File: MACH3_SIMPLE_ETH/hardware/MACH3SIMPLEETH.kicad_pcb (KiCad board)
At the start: 4 copper layers, 210 x 155 mm, 337 parts, among them J101 SENSORS / 24V IN, J201 USB-C, J202 SWD, J203 microSD, J301 HR911105A, J401 X axis, J402 Y axis, J403 Z axis, J404 A axis, J405 B axis, J406 C axis, J407 U axis, J408 V axis, J409 ENABLE, J501 LIMITS X Y Z A B C U V, J502 EST HLD RUN PRB, J503 THC AOK UP DN, J601 EXPANSION, J611 Relay A, J612 Relay B, J613 Relay C, J614 Relay D, J615 Relay E, J616 Relay F, J701 VFD, J801 RS485 A B GND, J802 HW ICSP, J803 MPG PENDANT, K601 JQC-3FF-024-1Z, K602 JQC-3FF-024-1Z, K603 JQC-3FF-024-1Z, K604 JQC-3FF-024-1Z, K605 JQC-3FF-024-1Z, K606 JQC-3FF-024-1Z, Q601 AO3400A, Q602 AO3400A, Q603 AO3400A, Q604 AO3400A, Q605 AO3400A, Q606 AO3400A, SW201 RESET, SW202 BOOTSEL, U101 LM2596S-5, U102 AP7361C-33E, U201 RP2350B, U202 W25Q128JVS, U203 USBLC6-2SC6, U301 W5500, U401 74ACT245, U402 74ACT245, U403 74ACT245, U501 PC847, U502 PC847, U503 PC847, U504 PC847, U601 MCP23017-E/SO, U701 74HCT14, U702 PC847, U703 B2412S-1WR3, U704 78L05, U705 LM358, U801 MAX3485ESA, U802 ATmega328P-AU, Y201 12MHz ABM8-272-T3, Y301 25MHz 18pF, Y801 8MHz

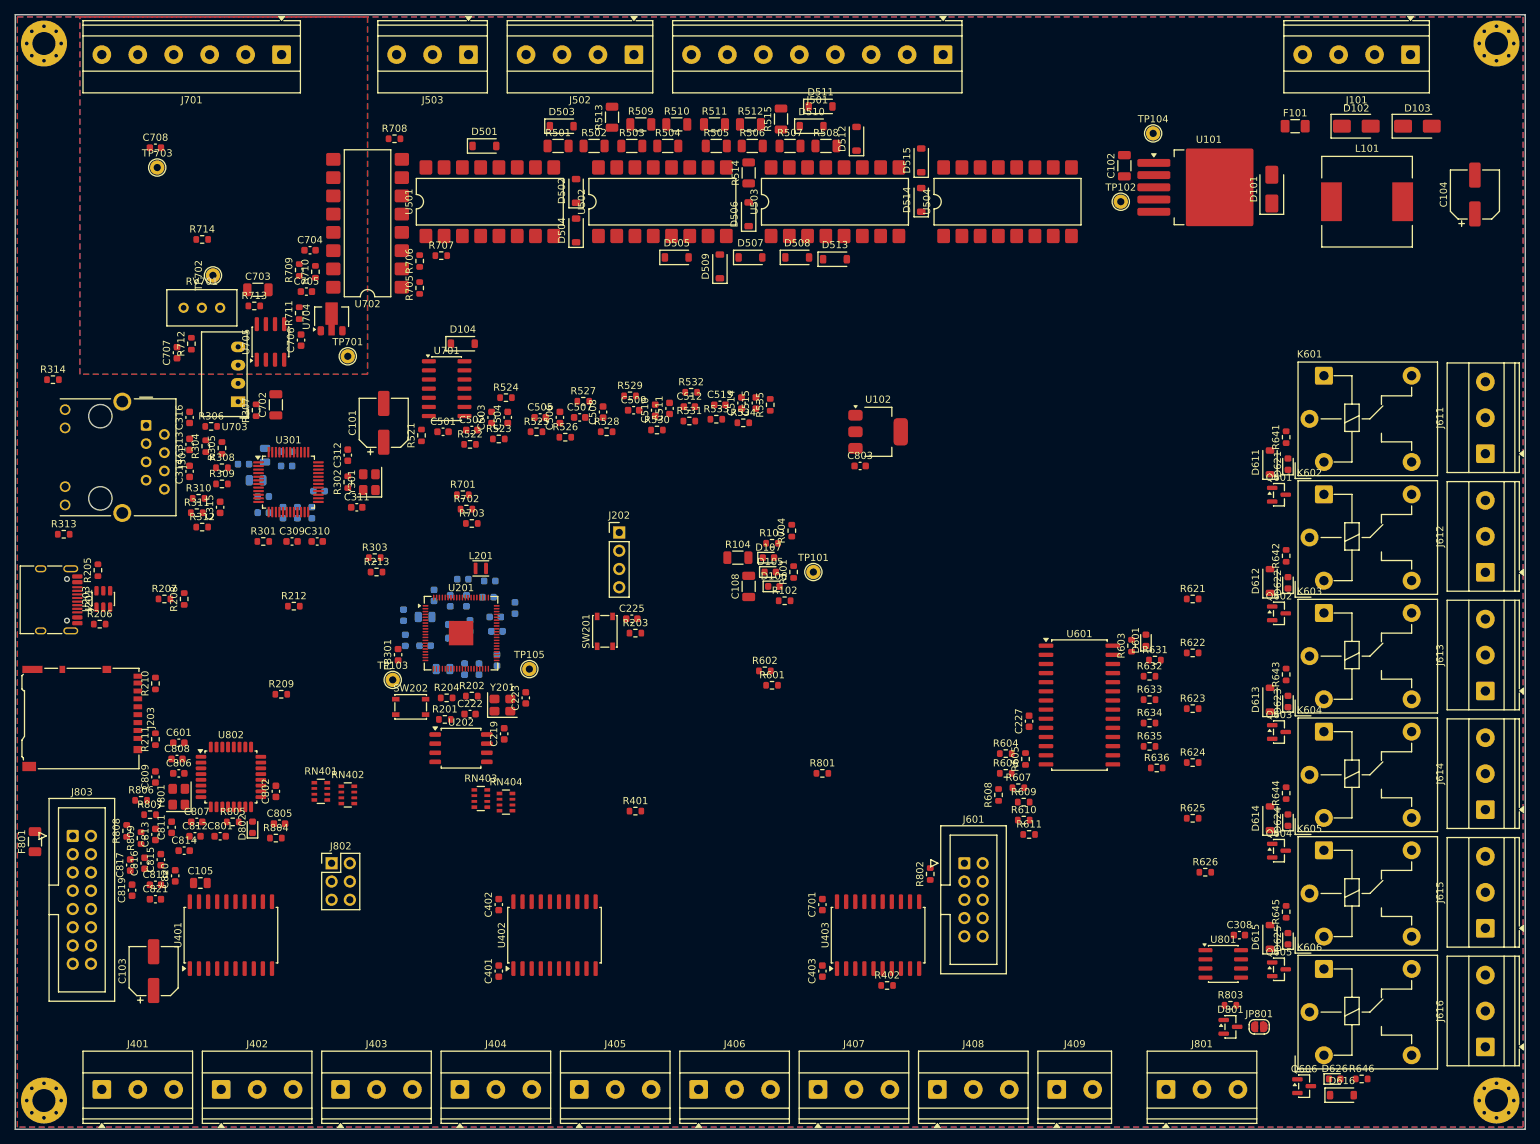
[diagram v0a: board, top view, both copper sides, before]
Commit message: MACH3-SIMPLE-ETH: routing pass 1 imported and filled
Freerouting pass 1 (board nets, VFD corner kept out): 1 h 40 min, 40
passes. After the zone fill 44 connections remain: 29 on the VFD side
(pass 2's job) and 15 others - 7 GND pins inside the RP2350B/W5500 fanout,
3 CHASSIS, 3 VBUS, 2 +3V3. Most of the 91 Freerouting reported were GND
pads that reach the ground pours once they are filled.

Co-Authored-By: Claude Opus 5.5 <noreply@anthropic.com>
Claude-Session: https://claude.ai/code/session_01MByiLT2xCcbGPkgCYQy33q
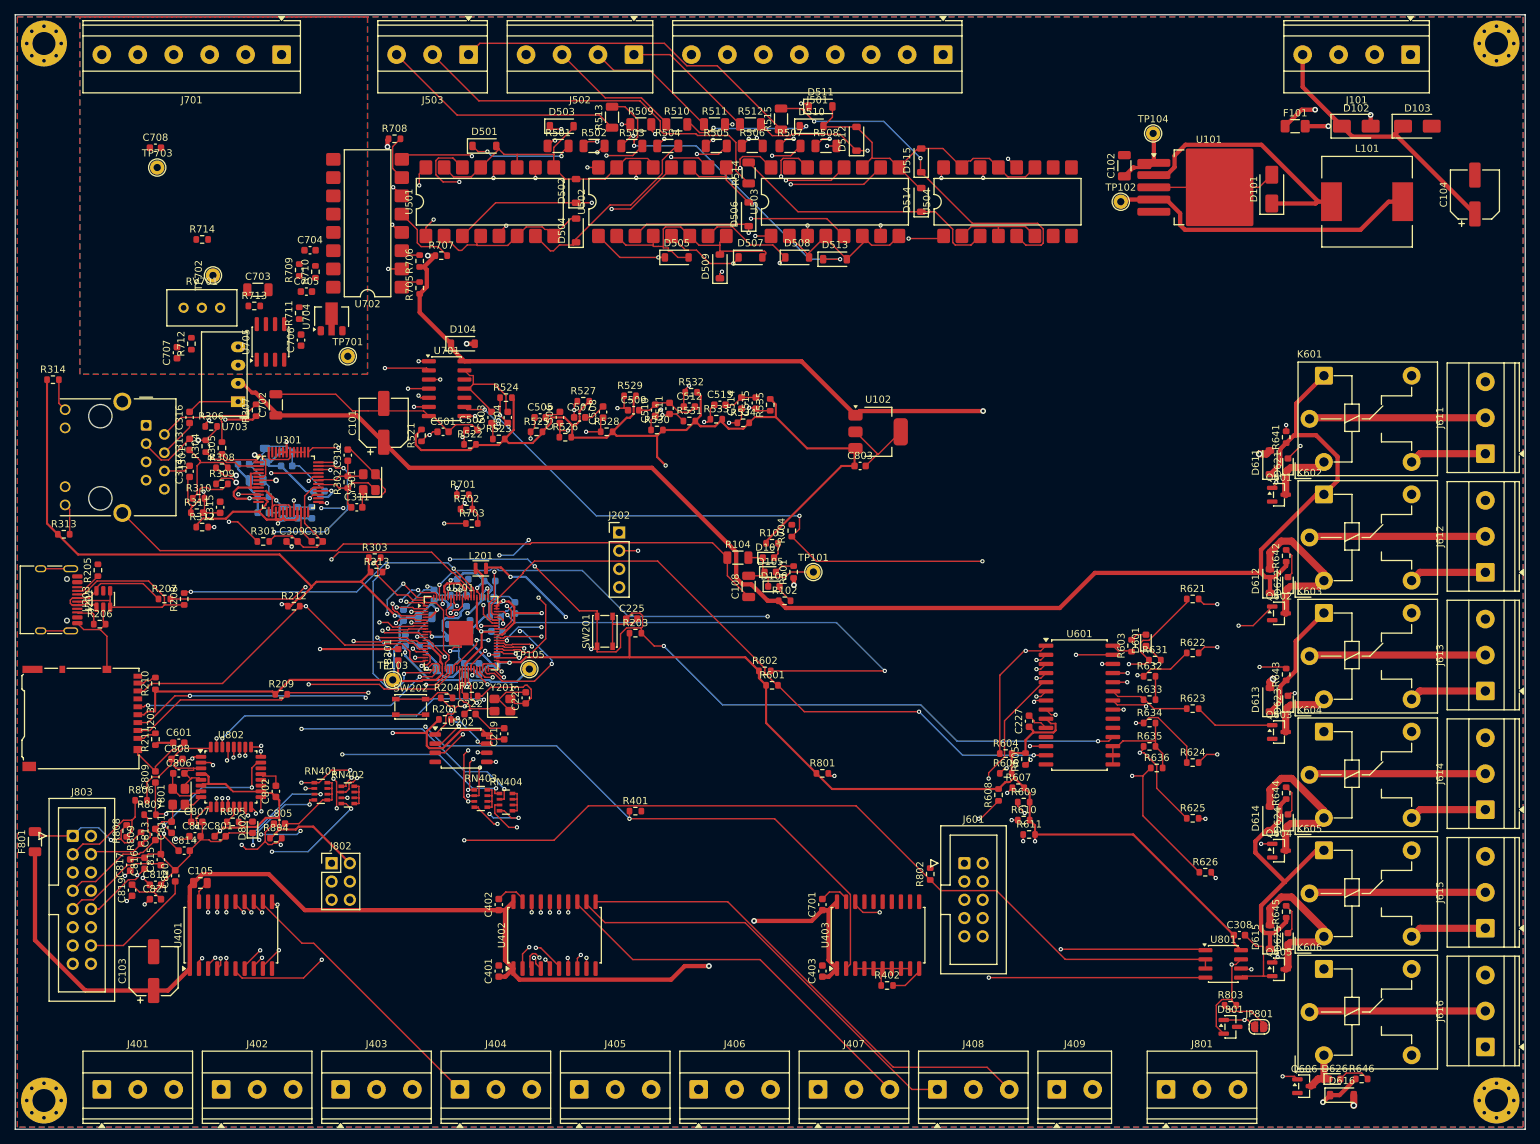
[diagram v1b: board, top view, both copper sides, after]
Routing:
- net +3V3: track 0.00 -> 693.7 mm, vias 0 -> 14
- net GND: track 0.00 -> 640.5 mm, vias 0 -> 3
- net V24: track 0.00 -> 482.2 mm, vias 0 -> 1
- net +5V: track 0.00 -> 452.5 mm, vias 0 -> 6
- net CHASSIS: track 0.00 -> 252.0 mm
- net NRST: track 0.00 -> 163.4 mm, vias 0 -> 7
- net RS485_DI: track 0.00 -> 155.4 mm, vias 0 -> 2
- net RS485_DE: track 0.00 -> 143.3 mm, vias 0 -> 2
- net RS485_RO: track 0.00 -> 143.2 mm, vias 0 -> 4
- net X_LIM: track 0.00 -> 112.0 mm, vias 0 -> 3
- net SP_AUX_IN: track 0.00 -> 107.7 mm, vias 0 -> 4
- net THC_DOWN: track 0.00 -> 105.7 mm, vias 0 -> 3
- net Y_LIM: track 0.00 -> 104.8 mm, vias 0 -> 4
- net THC_UP: track 0.00 -> 101.6 mm, vias 0 -> 4
- net ARC_OK: track 0.00 -> 101.0 mm, vias 0 -> 3
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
